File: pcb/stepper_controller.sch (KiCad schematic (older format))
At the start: 58 parts, among them P1 PWR_JACK_2.5x5.5, P10 HEADER_02X08_SMD, P11 HEADER_02X08_SMD, P2 HEADER_01X03_SMD_RA, P3 HEADER_01X03_SMD_RA, P4 HEADER_01X03_SMD_RA, P5 HEADER_01X03_SMD_RA, P6 HEADER_01X02_SMD_RA, P7 BNC_DOUBLE_RA, P8 HEADER_02X08_SMD, P9 HEADER_02X08_SMD, SW1 SPST_SLIDE_AS, U1 TLE7230R, U2 TLE7230R, U3 TLE7230R, U4 TLE7230R

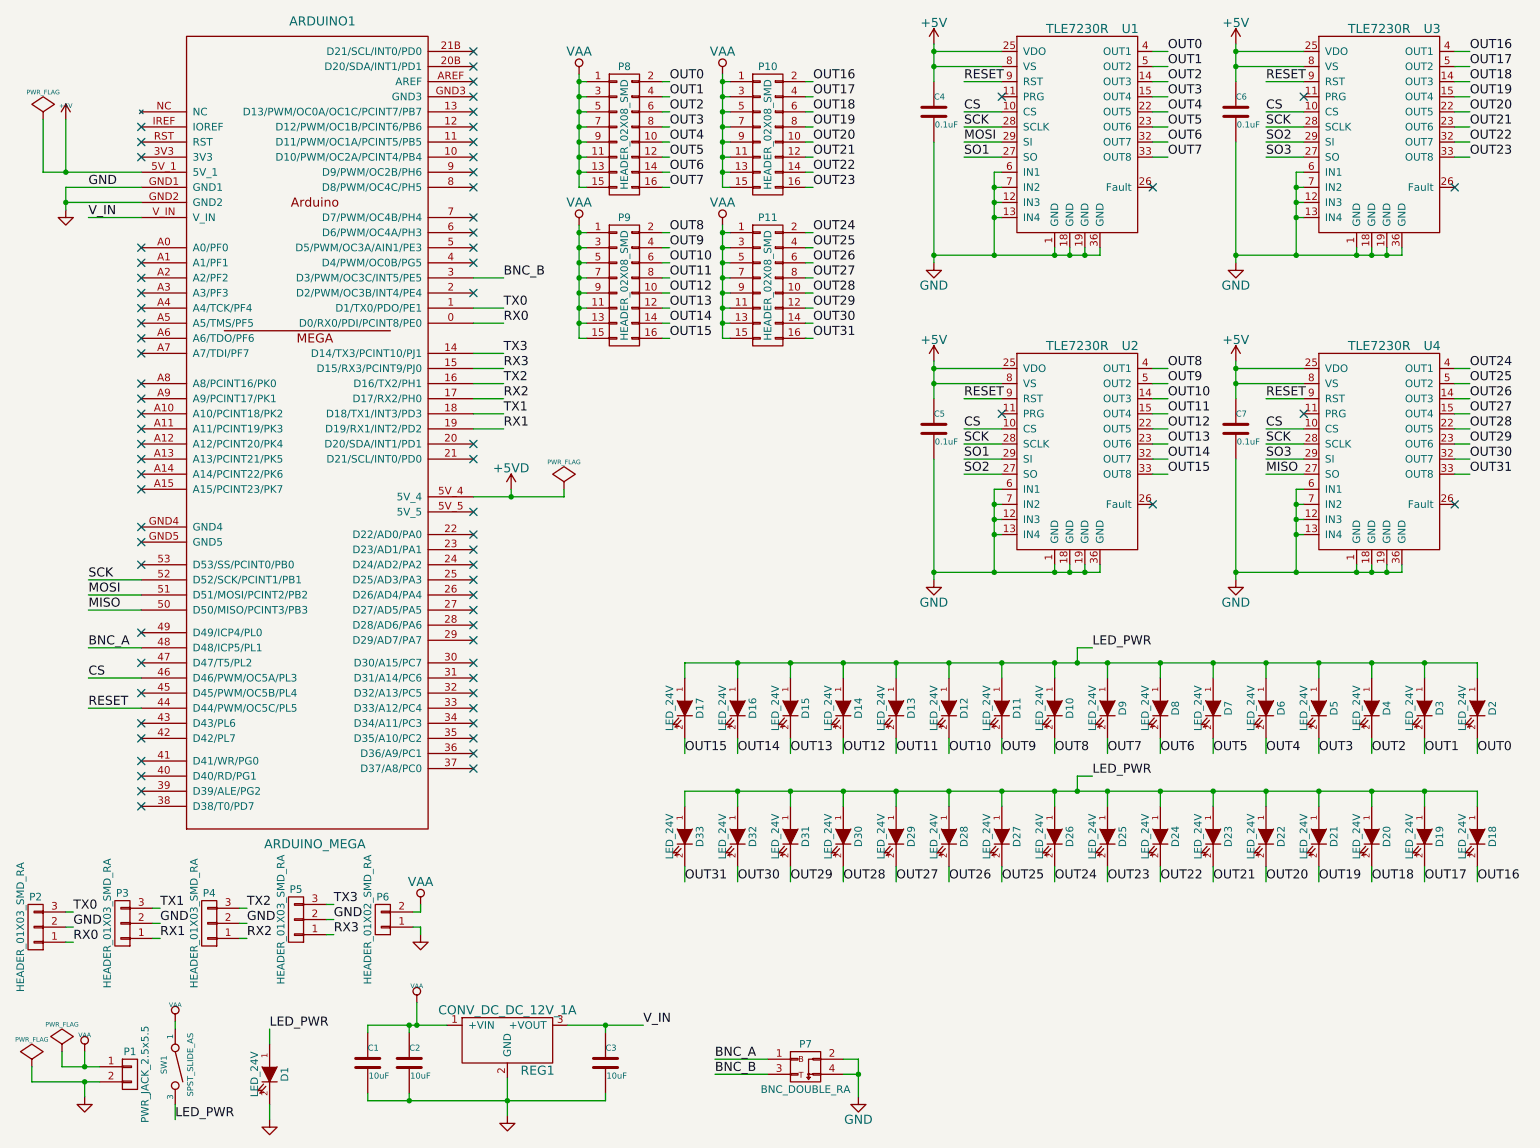
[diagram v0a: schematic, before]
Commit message: Progress towards pcb 1.0.
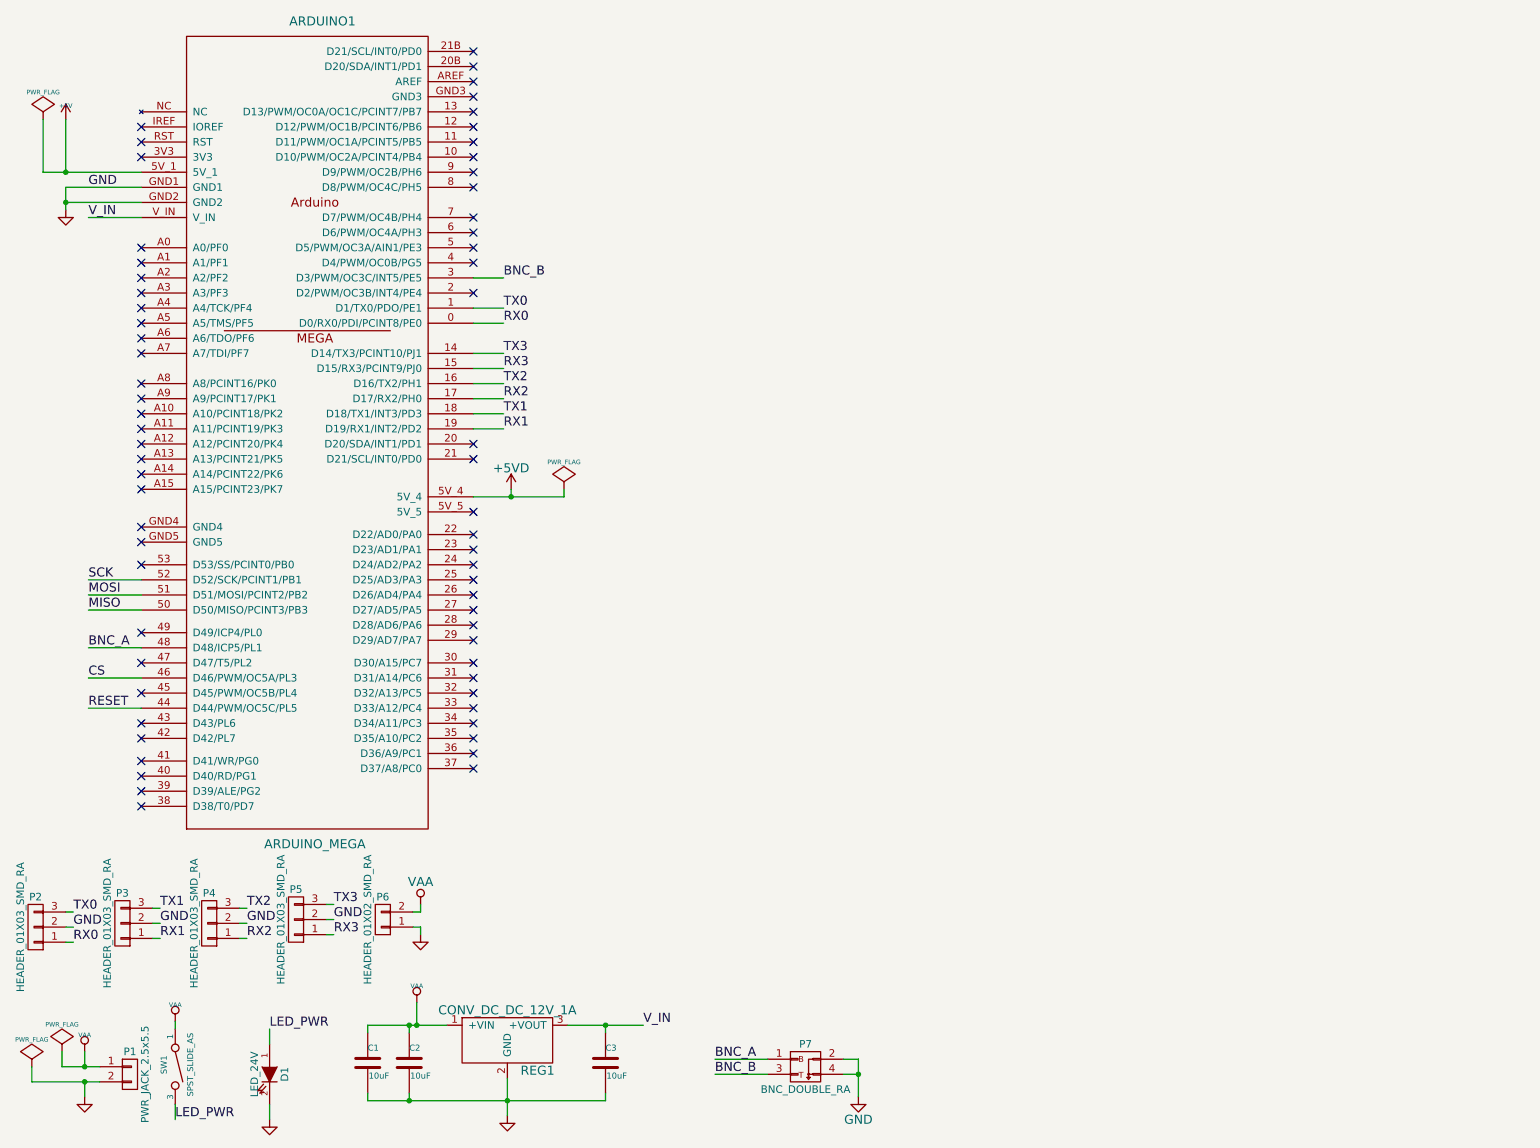
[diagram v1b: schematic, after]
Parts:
- removed C4, C5, C6, C7: 0.1uF, stepper_controller:SM1210, symbol 0.1uF
- removed D10, D11, D12, D13, D14, D15, D16, D17, D18, D19, D2, D20, D21, D22, D23, D24, D25, D26, D27, D28, D29, D3, D30, D31, D32, D33, D4, D5, D6, D7, D8, D9: LED_24V, stepper_controller:LED_555-3XXX, symbol LED_24V
- removed P10, P11, P8, P9: HEADER_02X08_SMD, stepper_controller:HEADER_02x08_SMD, symbol HEADER_02X08_SMD
- removed U1, U2, U3, U4: TLE7230R, stepper_controller:PG-DSO-36, symbol TLE7230R
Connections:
- no-connect marks 73 -> 65
